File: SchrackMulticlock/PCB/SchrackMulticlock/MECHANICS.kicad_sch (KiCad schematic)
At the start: 18 parts, among them SW2 SW_Push, SW3 SW_Push, SW4 SW_Push, SW5 SW_Push, SW6 SW_Push

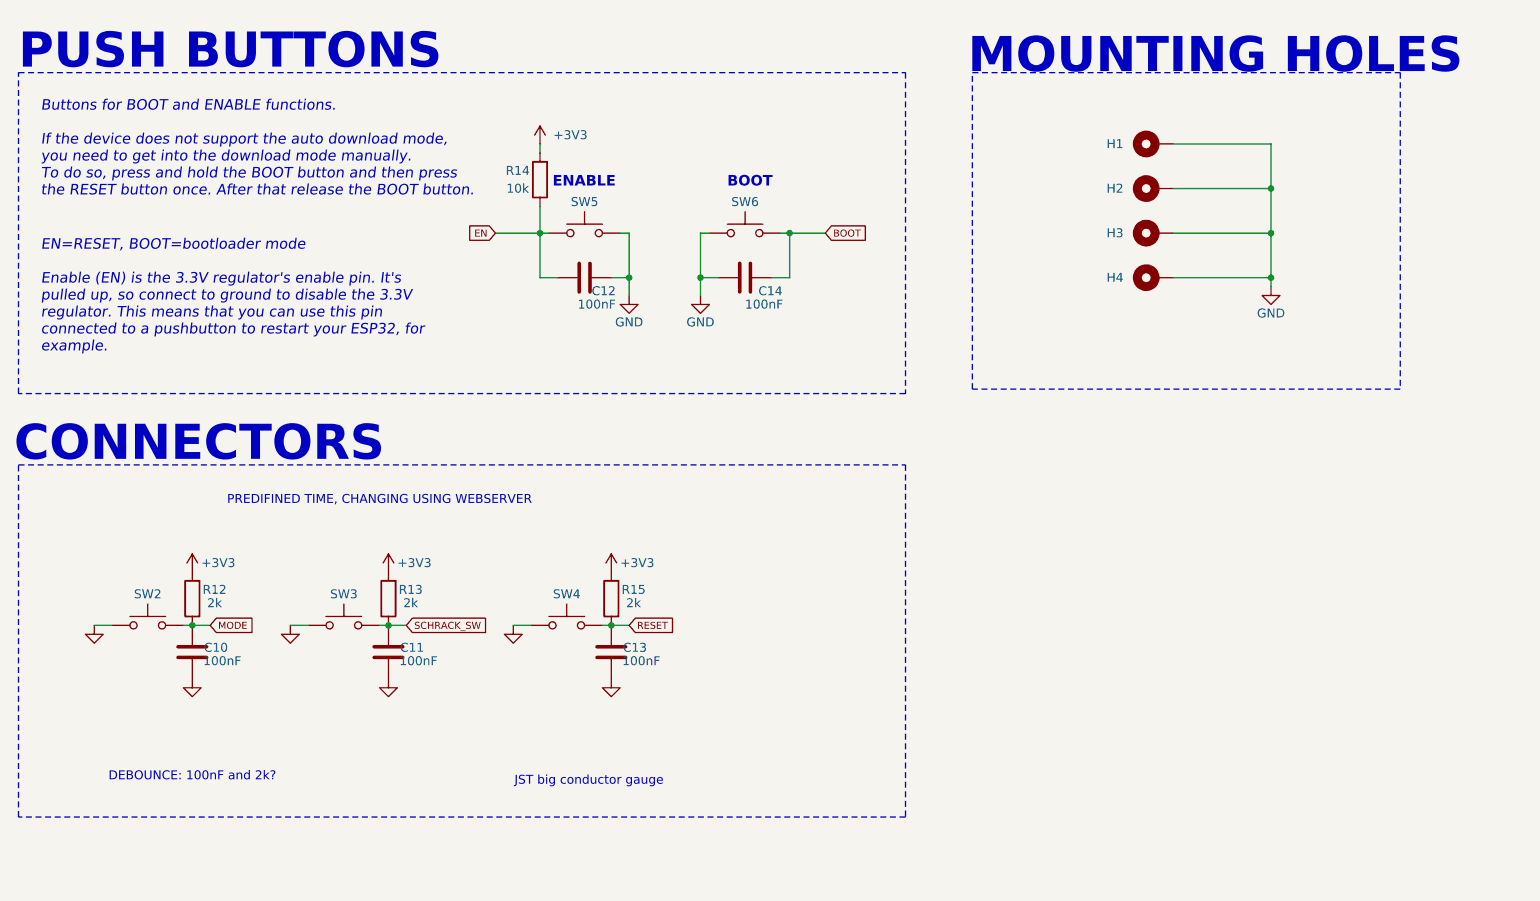
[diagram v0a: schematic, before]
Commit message: schrack multiclock schematic update
Just regular updates
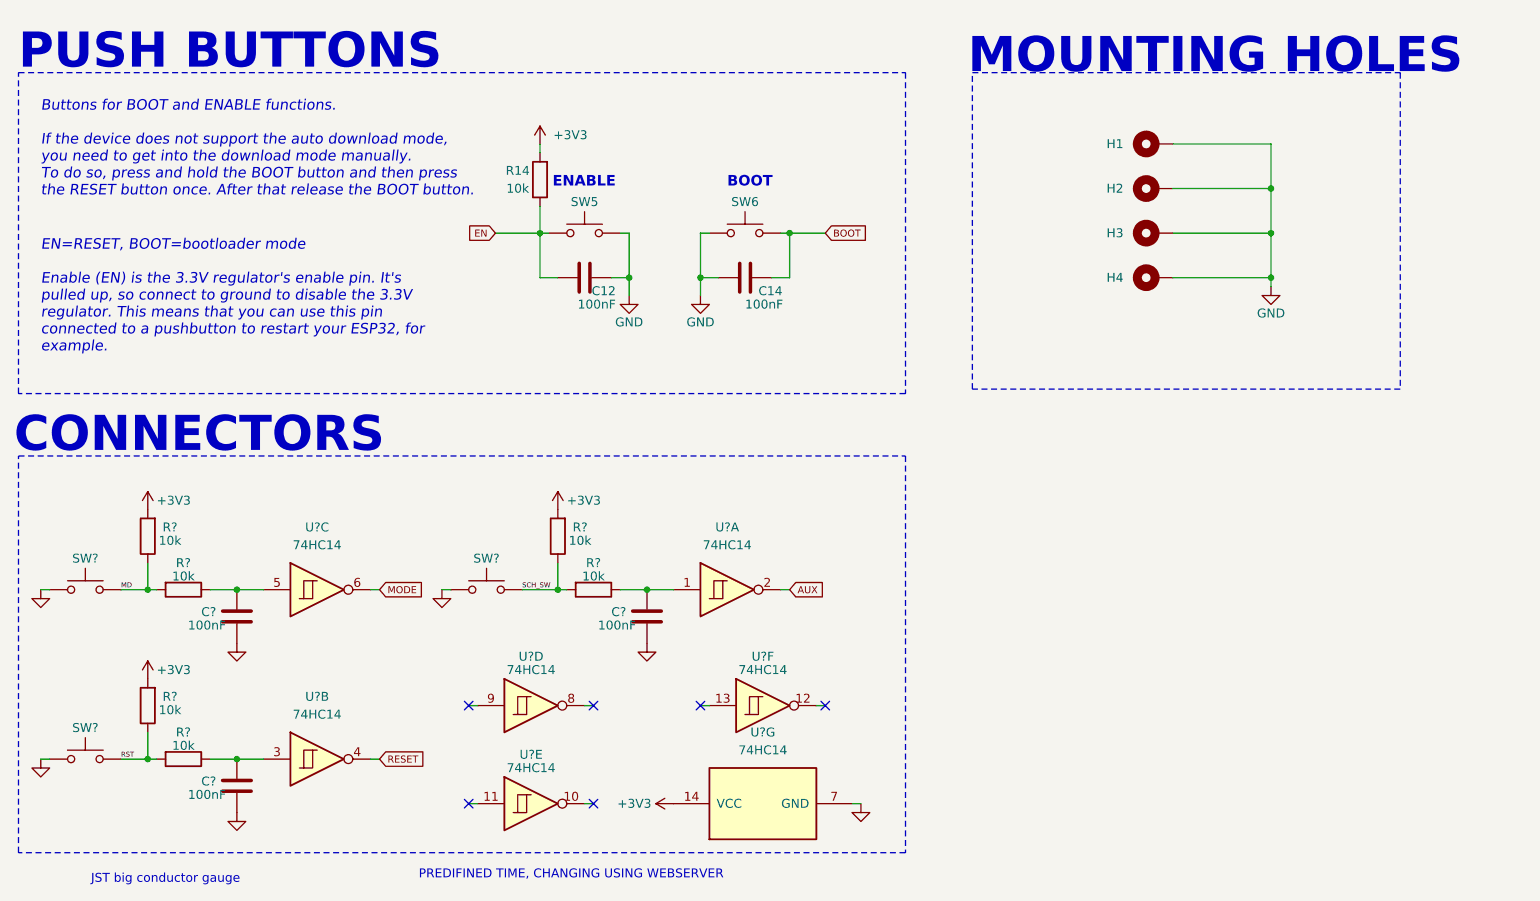
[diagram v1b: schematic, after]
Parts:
- removed C10, C11, C13: 100nF, Capacitor_SMD:C_0805_2012Metric_Pad1.18x1.45mm_HandSolder, symbol Device:C
- removed R12, R13, R15: 2k, Resistor_SMD:R_0805_2012Metric_Pad1.20x1.40mm_HandSolder, symbol Device:R
- removed SW2, SW3, SW4: SW_Push, Connector_JST:JST_XH_B2B-XH-A_1x02_P2.50mm_Vertical, symbol Switch:SW_Push
- added C? (x3): 100nF, Capacitor_SMD:C_0805_2012Metric_Pad1.18x1.45mm_HandSolder, symbol Device:C
- added R? (x6): 10k, Resistor_SMD:R_0805_2012Metric_Pad1.20x1.40mm_HandSolder, symbol Device:R
- added SW? (x3): SW_Push, Connector_JST:JST_XH_B2B-XH-A_1x02_P2.50mm_Vertical, symbol Switch:SW_Push
- added U? (x7): 74HC14, Package_SO:SOIC-14_3.9x8.7mm_P1.27mm, symbol 74xx:74HC14
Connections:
- net +3V3: now also R?.2, R?.2, R?.2, U?.14 (VCC)
- net GND: now also C?.1, C?.1, C?.1, SW?.1, SW?.1, SW?.1, U?.7 (GND)
- net MODE: now also U?.6
- net RESET: now also U?.4
- new net: C?.2, R?.1, U?.3
- new net: C?.2, R?.1, U?.5
- new net: C?.2, R?.1, U?.1
- new net AUX: U?.2
- new net MD: R?.1, R?.2, SW?.2
- new net RST: R?.1, R?.2, SW?.2
- new net SCH_SW: R?.1, R?.2, SW?.2
- no-connect marks 0 -> 6
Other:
- note removed: "DEBOUNCE: 100nF and 2k?"
